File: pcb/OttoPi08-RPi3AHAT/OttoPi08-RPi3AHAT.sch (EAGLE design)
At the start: 39 parts

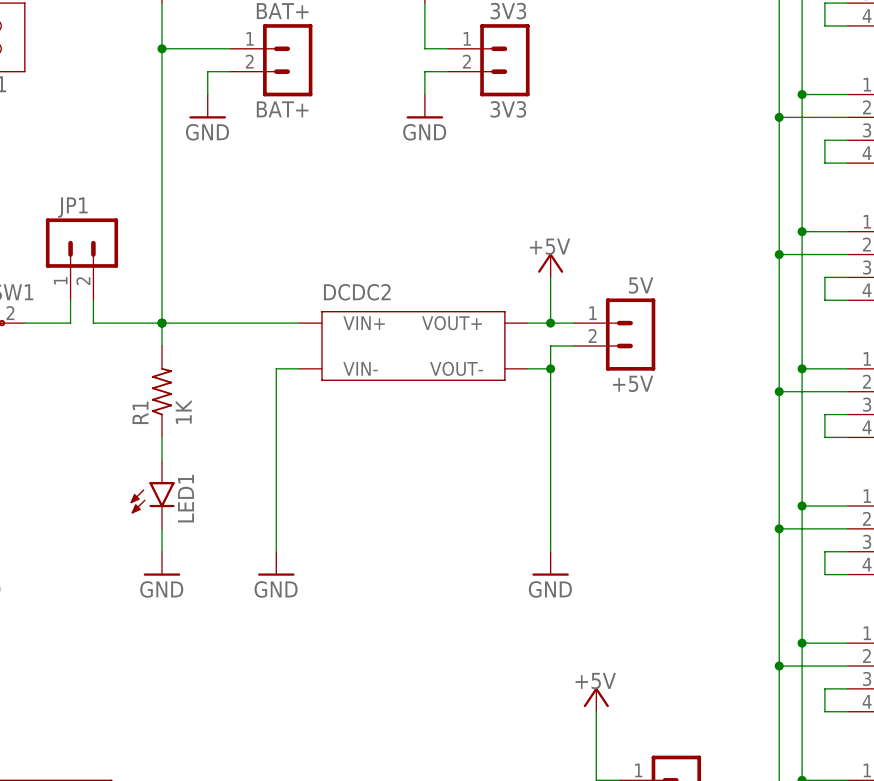
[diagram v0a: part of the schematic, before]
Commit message: UPD: pcb/OttoPi08-RPi3AHAT
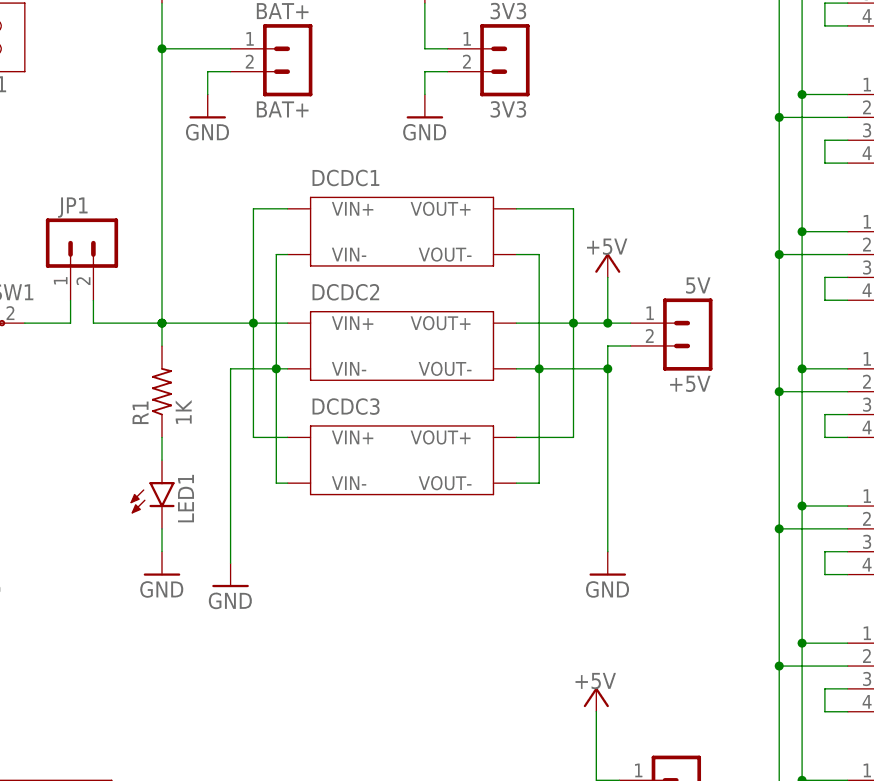
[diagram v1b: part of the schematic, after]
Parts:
- added DCDC1: (no value), ytani1:DCDC-MT3608-MOD
- added DCDC3: (no value), ytani1:DCDC-MT3608-MODUSB
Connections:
- net +5V: now also DCDC1.VOUT+, DCDC3.VOUT+
- net BAT+: now also DCDC1.VIN+, DCDC3.VIN+
- net GND: now also DCDC1.VIN-, DCDC1.VOUT-, DCDC3.VIN-, DCDC3.VOUT-
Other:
- moved on the sheet: +5V, DCDC2
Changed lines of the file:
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@@
 <part name="SV10" library="ytani1" deviceset="PINHEAD-MA04-1" device="" package3d_urn="urn:adsk.eagle:package:8337/1"/>
 <part name="DCDC2" library="ytani1" deviceset="DCDC-SX1308-MOD1" device=""/>
+<part name="DCDC1" library="ytani1" library_urn="urn:adsk.eagle:library:30941153" deviceset="DCDC-MT3608-MOD" device="" package3d_urn="urn:adsk.eagle:package:23610132/1"/>
+<part name="DCDC3" library="ytani1" library_urn="urn:adsk.eagle:library:30941153" deviceset="DCDC-MT3608-MOD" device="USB" package3d_urn="urn:adsk.eagle:package:23610144/1"/>
 </parts>
 <sheets>
@@
 </plain>
 <instances>
-<instance part="P+2" gate="1" x="43.18" y="152.4" smashed="yes">
-<attribute name="VALUE" x="40.64" y="152.4" size="1.778" layer="96"/>
+<instance part="P+2" gate="1" x="49.53" y="152.4" smashed="yes">
+<attribute name="VALUE" x="46.99" y="152.4" size="1.778" layer="96"/>
 </instance>
 <instance part="P+4" gate="VCC" x="0" y="182.88" smashed="yes">
 <attribute name="VALUE" x="-2.54" y="182.88" size="1.778" layer="96"/>
 </instance>
-<instance part="GND2" gate="1" x="12.7" y="116.84" smashed="yes">
-<attribute name="VALUE" x="10.16" y="114.3" size="1.778" layer="96"/>
+<instance part="GND2" gate="1" x="7.62" y="115.57" smashed="yes">
+<attribute name="VALUE" x="5.08" y="113.03" size="1.778" layer="96"/>
 </instance>
 <instance part="GND3" gate="1" x="-50.8" y="35.56" smashed="yes">
@@
 <attribute name="VALUE" x="150.876" y="63.119" size="1.778" layer="96" rot="R180"/>
 </instance>
-<instance part="GND5" gate="1" x="43.18" y="116.84" smashed="yes">
-<attribute name="VALUE" x="40.64" y="114.3" size="1.778" layer="96"/>
+<instance part="GND5" gate="1" x="49.53" y="116.84" smashed="yes">
+<attribute name="VALUE" x="46.99" y="114.3" size="1.778" layer="96"/>
 </instance>
 <instance part="BAT+" gate="G$1" x="15.24" y="175.26" smashed="yes" rot="R180">
@@
 <attribute name="NAME" x="16.51" y="169.418" size="1.778" layer="95" rot="R180"/>
 </instance>
-<instance part="+5V" gate="G$1" x="53.34" y="144.78" smashed="yes" rot="R180">
-<attribute name="VALUE" x="54.61" y="149.86" size="1.778" layer="96" rot="R180"/>
-<attribute name="NAME" x="54.61" y="138.938" size="1.778" layer="95" rot="R180"/>
+<instance part="+5V" gate="G$1" x="59.69" y="144.78" smashed="yes" rot="R180">
+<attribute name="VALUE" x="60.96" y="149.86" size="1.778" layer="96" rot="R180"/>
+<attribute name="NAME" x="60.96" y="138.938" size="1.778" layer="95" rot="R180"/>
 </instance>
 <instance part="JP1" gate="G$1" x="-10.16" y="154.94" smashed="yes" rot="R270">
@@
 <attribute name="NAME" x="85.852" y="46.99" size="1.778" layer="95" rot="R270"/>
 </instance>
-<instance part="DCDC2" gate="G$1" x="27.94" y="142.24" smashed="yes">
-<attribute name="NAME" x="17.78" y="147.32" size="1.778" layer="95"/>
-<attribute name="VALUE" x="38.32" y="143.24" size="1.4224" layer="96"/>
+<instance part="DCDC2" gate="G$1" x="26.67" y="142.24" smashed="yes">
+<attribute name="NAME" x="16.51" y="147.32" size="1.778" layer="95"/>
+<attribute name="VALUE" x="37.05" y="143.24" size="1.4224" layer="96"/>
+</instance>
+<instance part="DCDC1" gate="G$1" x="26.67" y="154.94" smashed="yes">
+<attribute name="NAME" x="16.51" y="160.02" size="1.778" layer="95"/>
+<attribute name="VALUE" x="37.05" y="155.94" size="1.4224" layer="96"/>
+</instance>
+<instance part="DCDC3" gate="G$1" x="26.67" y="129.54" smashed="yes">
+<attribute name="NAME" x="16.51" y="134.62" size="1.778" layer="95"/>
+<attribute name="VALUE" x="37.05" y="130.54" size="1.4224" layer="96"/>
 </instance>
 </instances>
@@
 </segment>
 <segment>
-<wire x1="12.7" y1="119.38" x2="12.7" y2="139.7" width="0.1524" layer="91"/>
+<wire x1="7.62" y1="118.11" x2="7.62" y2="139.7" width="0.1524" layer="91"/>
 <pinref part="GND2" gate="1" pin="GND"/>
-<wire x1="15.24" y1="139.7" x2="12.7" y2="139.7" width="0.1524" layer="91"/>
+<wire x1="13.97" y1="139.7" x2="12.7" y2="139.7" width="0.1524" layer="91"/>
 <pinref part="DCDC2" gate="G$1" pin="VIN-"/>
+<pinref part="DCDC1" gate="G$1" pin="VIN-"/>
+<wire x1="12.7" y1="139.7" x2="7.62" y2="139.7" width="0.1524" layer="91"/>
+<wire x1="13.97" y1="152.4" x2="12.7" y2="152.4" width="0.1524" layer="91"/>
+<wire x1="12.7" y1="152.4" x2="12.7" y2="139.7" width="0.1524" layer="91"/>
+<junction x="12.7" y="139.7"/>
+<pinref part="DCDC3" gate="G$1" pin="VIN-"/>
+<wire x1="12.7" y1="139.7" x2="12.7" y2="127" width="0.1524" layer="91"/>
+<wire x1="12.7" y1="127" x2="13.97" y2="127" width="0.1524" layer="91"/>
 </segment>
 <segment>
@@
 </segment>
 <segment>
-<wire x1="43.18" y1="142.24" x2="43.18" y2="139.7" width="0.1524" layer="91"/>
-<wire x1="45.72" y1="142.24" x2="43.18" y2="142.24" width="0.1524" layer="91"/>
-<wire x1="40.64" y1="139.7" x2="43.18" y2="139.7" width="0.1524" layer="91"/>
+<wire x1="49.53" y1="142.24" x2="49.53" y2="139.7" width="0.1524" layer="91"/>
+<wire x1="52.07" y1="142.24" x2="49.53" y2="142.24" width="0.1524" layer="91"/>
+<wire x1="39.37" y1="139.7" x2="41.91" y2="139.7" width="0.1524" layer="91"/>
 <pinref part="+5V" gate="G$1" pin="2"/>
 <pinref part="DCDC2" gate="G$1" pin="VOUT-"/>
 <pinref part="GND5" gate="1" pin="GND"/>
-<wire x1="43.18" y1="119.38" x2="43.18" y2="139.7" width="0.1524" layer="91"/>
-<junction x="43.18" y="139.7"/>
+<wire x1="41.91" y1="139.7" x2="49.53" y2="139.7" width="0.1524" layer="91"/>
+<wire x1="49.53" y1="119.38" x2="49.53" y2="139.7" width="0.1524" layer="91"/>
+<junction x="49.53" y="139.7"/>
+<pinref part="DCDC1" gate="G$1" pin="VOUT-"/>
+<wire x1="39.37" y1="152.4" x2="41.91" y2="152.4" width="0.1524" layer="91"/>
+<wire x1="41.91" y1="152.4" x2="41.91" y2="139.7" width="0.1524" layer="91"/>
+<junction x="41.91" y="139.7"/>
+<pinref part="DCDC3" gate="G$1" pin="VOUT-"/>
+<wire x1="41.91" y1="139.7" x2="41.91" y2="127" width="0.1524" layer="91"/>
+<wire x1="41.91" y1="127" x2="39.37" y2="127" width="0.1524" layer="91"/>
 </segment>
 </net>
@@
 <pinref part="BAT+" gate="G$1" pin="1"/>
 <pinref part="DCDC2" gate="G$1" pin="VIN+"/>
-<wire x1="15.24" y1="144.78" x2="0" y2="144.78" width="0.1524" layer="91"/>
+<wire x1="13.97" y1="144.78" x2="10.16" y2="144.78" width="0.1524" layer="91"/>
+<pinref part="DCDC3" gate="G$1" pin="VIN+"/>
+<wire x1="10.16" y1="144.78" x2="0" y2="144.78" width="0.1524" layer="91"/>
+<wire x1="13.97" y1="132.08" x2="10.16" y2="132.08" width="0.1524" layer="91"/>
+<wire x1="10.16" y1="132.08" x2="10.16" y2="144.78" width="0.1524" layer="91"/>
+<junction x="10.16" y="144.78"/>
+<pinref part="DCDC1" gate="G$1" pin="VIN+"/>
+<wire x1="13.97" y1="157.48" x2="10.16" y2="157.48" width="0.1524" layer="91"/>
+<wire x1="10.16" y1="157.48" x2="10.16" y2="144.78" width="0.1524" layer="91"/>
 </segment>
 <segment>
@@
 <segment>
 <pinref part="P+2" gate="1" pin="+5V"/>
-<wire x1="43.18" y1="149.86" x2="43.18" y2="144.78" width="0.1524" layer="91"/>
-<wire x1="43.18" y1="144.78" x2="45.72" y2="144.78" width="0.1524" layer="91"/>
-<wire x1="40.64" y1="144.78" x2="43.18" y2="144.78" width="0.1524" layer="91"/>
-<junction x="43.18" y="144.78"/>
+<wire x1="49.53" y1="149.86" x2="49.53" y2="144.78" width="0.1524" layer="91"/>
+<wire x1="49.53" y1="144.78" x2="52.07" y2="144.78" width="0.1524" layer="91"/>
+<wire x1="39.37" y1="144.78" x2="45.72" y2="144.78" width="0.1524" layer="91"/>
+<junction x="49.53" y="144.78"/>
 <pinref part="+5V" gate="G$1" pin="1"/>
 <pinref part="DCDC2" gate="G$1" pin="VOUT+"/>
-</segment>
-<segment>
+<pinref part="DCDC1" gate="G$1" pin="VOUT+"/>
+<wire x1="45.72" y1="144.78" x2="49.53" y2="144.78" width="0.1524" layer="91"/>
+<wire x1="39.37" y1="157.48" x2="45.72" y2="157.48" width="0.1524" layer="91"/>
+<wire x1="45.72" y1="157.48" x2="45.72" y2="144.78" width="0.1524" layer="91"/>
+<junction x="45.72" y="144.78"/>
+<pinref part="DCDC3" gate="G$1" pin="VOUT+"/>
+<wire x1="39.37" y1="132.08" x2="45.72" y2="132.08" width="0.1524" layer="91"/>
+<wire x1="45.72" y1="132.08" x2="45.72" y2="144.78" width="0.1524" layer="91"/>
+</segment>
+<segment>
